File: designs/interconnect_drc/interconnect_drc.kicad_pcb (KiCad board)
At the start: 2 copper layers, 90.7 x 60.5 mm, 2 parts

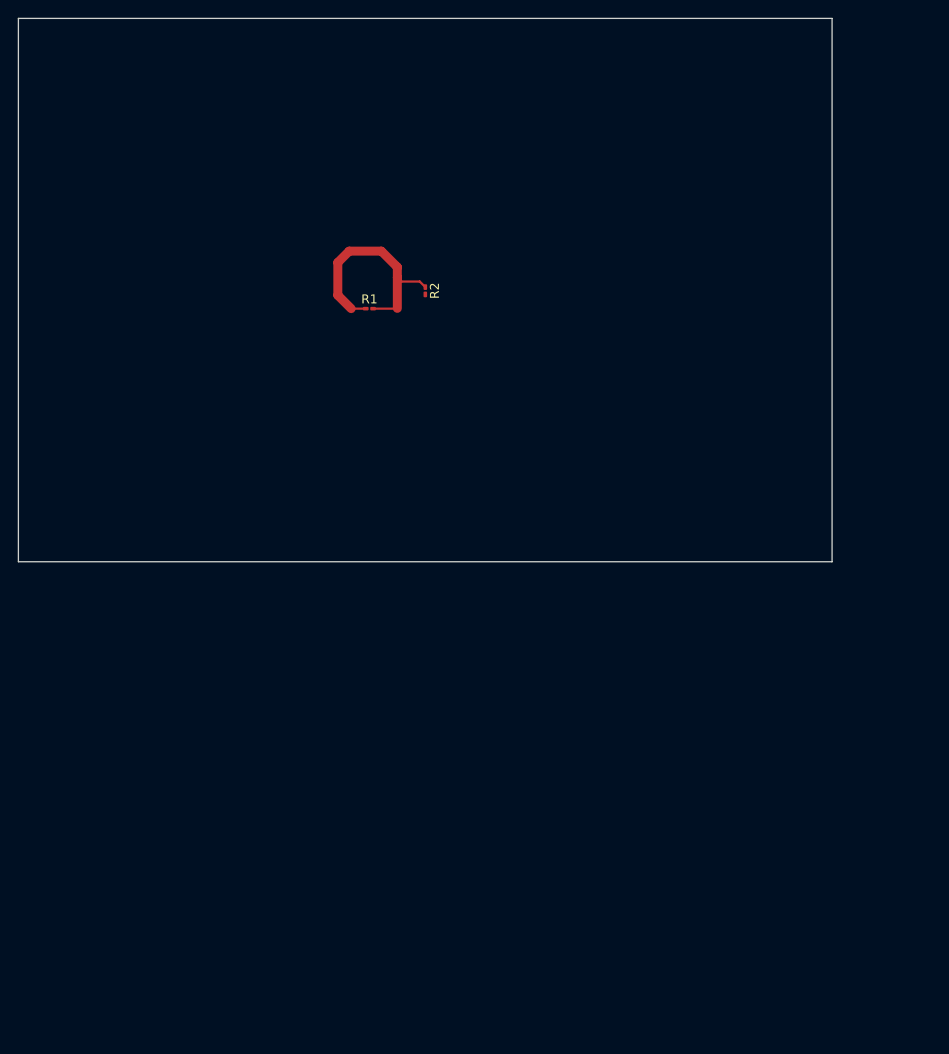
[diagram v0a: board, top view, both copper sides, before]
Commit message: Rename to tc6
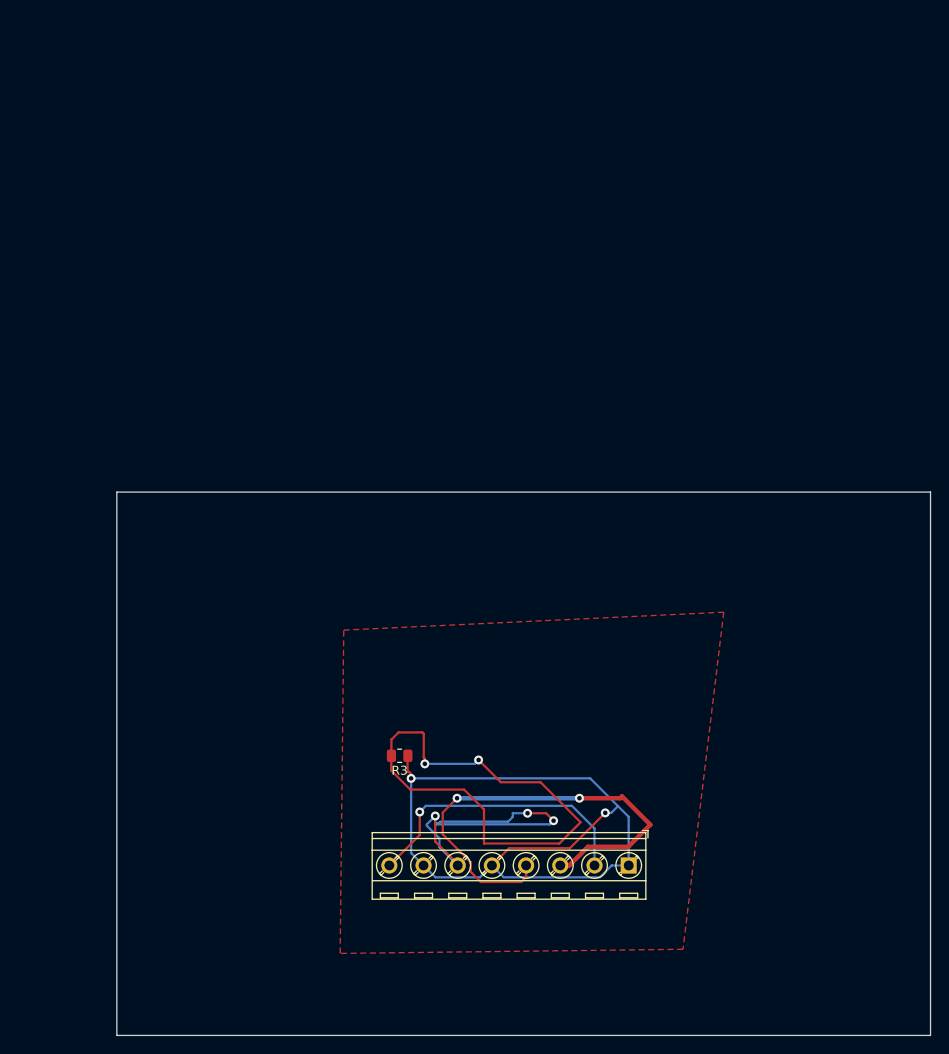
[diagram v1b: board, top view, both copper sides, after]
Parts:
- removed R1, R2: R_Small, Resistor_SMD:R_0201_0603Metric_Pad0.64x0.40mm_HandSolder
- added J1: Screw_Terminal_01x08, Project:TerminalBlock_Phoenix_MKDS_1727078_1x08_P3.81mm_Horizontal, F.Cu at (155.1, 146.1)
- added R3: R_Small, Resistor_SMD:R_0805_2012Metric, F.Cu at (129.5, 133.8)
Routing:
- net GND: track 0.00 -> 86.3 mm, vias 0 -> 2
- net +3V3: track 0.00 -> 58.9 mm, vias 0 -> 2
- net Net-(J1-Pin_3): track 0.00 -> 53.2 mm, vias 0 -> 2
- net Net-(J1-Pin_2): track 0.00 -> 32.3 mm, vias 0 -> 1
- net (no net): track 0.00 -> 27.7 mm, vias 0 -> 2
- net Net-(R1-Pad1): track 26.2 -> 0.00 mm
- net unconnected-(J1-Pin_6-Pad6): track 0.00 -> 13.2 mm, vias 0 -> 1
- added copper zone on F.Cu, net +3V3
